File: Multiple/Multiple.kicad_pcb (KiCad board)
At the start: 2 copper layers, 23.1 x 128.4 mm, 17 parts

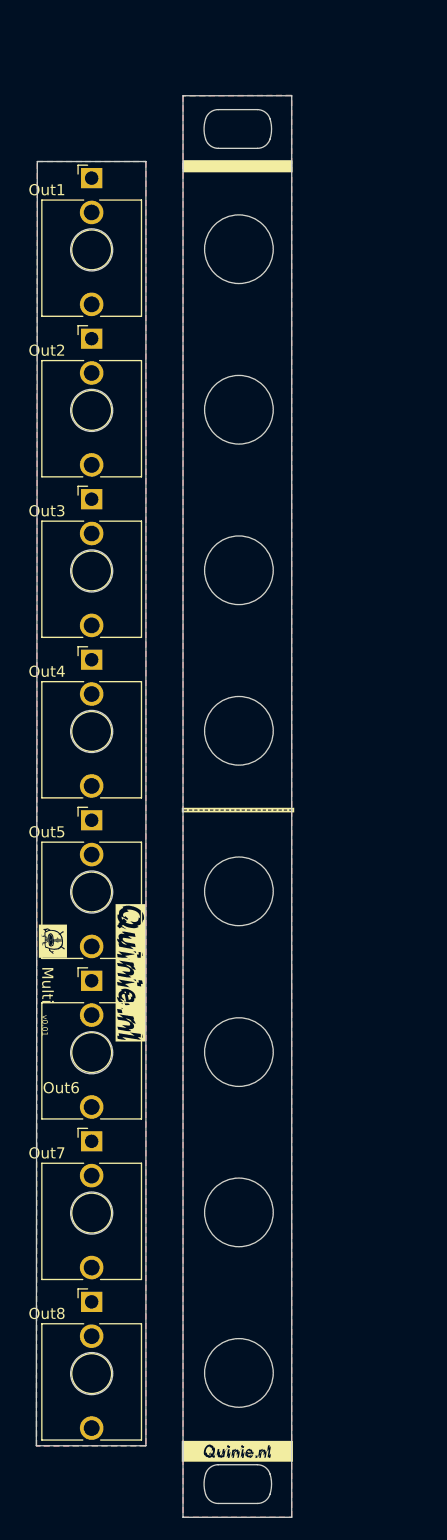
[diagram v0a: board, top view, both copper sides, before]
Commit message: Updates
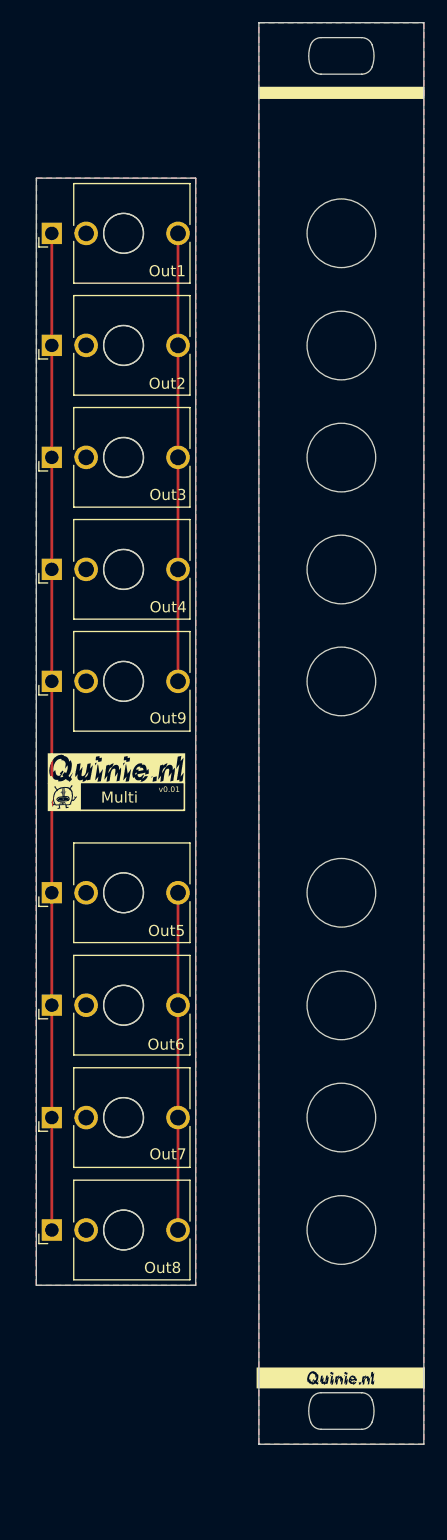
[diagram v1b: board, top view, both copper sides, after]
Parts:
- removed the kibuzzard-63663374 at (30.5, 108.9)
- removed the kibuzzard-63663374 at (37.6, 108.9)
- removed the kibuzzard-63663374 at (50.6, 108.7)
- removed the kibuzzard-63729A5C at (37.5, 111.8)
- removed the kibuzzard-63729A5C at (30.5, 111.8)
- removed the kibuzzard-63729A5C at (43.6, 111.5)
- removed kibuzzard-6564E26E: G***, kibuzzard-6564E26E
- removed kibuzzard-6564E2EE: G***, kibuzzard-6564E2EE
- removed kibuzzard-6564E9E6: G***, kibuzzard-6564E9E6
- added Out9: AudioJack2_SwitchT, Connector_Audio:Jack_3.5mm_QingPu_WQP-PJ398SM_Vertical_CircularHoles, F.Cu at (30.4, 85.5)
- added REF**: ESD-Logo_6.6x6mm_SilkScreen, Symbol:ESD-Logo_6.6x6mm_SilkScreen, B.Cu at (60.2, 109.6)
- added REF**: KiCad-Logo2_5mm_SilkScreen, Symbol:KiCad-Logo2_5mm_SilkScreen, B.Cu at (52.1, 95.0)
- added REF**: WEEE-Logo_4.2x6mm_SilkScreen, Symbol:WEEE-Logo_4.2x6mm_SilkScreen, B.Cu at (58.6, 91.4)
- added REF**: OSHW-Logo2_7.3x6mm_SilkScreen, Symbol:OSHW-Logo2_7.3x6mm_SilkScreen, B.Cu at (58.6, 97.5)
- added kibuzzard-63663374: G***, kibuzzard-63663374, F.Cu at (31.5, 95.9)
- added kibuzzard-63663374: G***, kibuzzard-63663374, B.Cu at (40.7, 95.7)
- added kibuzzard-63729A5C: G***, kibuzzard-63729A5C, F.Cu at (36.2, 93.3)
- added kibuzzard-63729A5C: G***, kibuzzard-63729A5C, B.Cu at (36.0, 93.1)
- added kibuzzard-656B6089: G***, kibuzzard-656B6089, F.Cu at (56.6, 146.1)
- added kibuzzard-656B60C2: G***, kibuzzard-656B60C2, F.Cu at (56.5, 148.4)
- added kibuzzard-656B617B: G***, kibuzzard-656B617B, B.Cu at (56.5, 38.1)
- moved Out4 8.92 mm to (30.4, 75.3), turned to 90 degrees
- moved Out5 7.47 mm to (30.4, 104.5), turned to 90 degrees
- moved Out8 7.42 mm to (30.4, 135.0), turned to 90 degrees
- moved Out1 6.15 mm to (30.4, 45.0), turned to 90 degrees
- moved Out3 5.22 mm to (30.4, 65.2), turned to 90 degrees
- moved Out6 4.22 mm to (30.4, 114.7), turned to 90 degrees
- moved Out7 4.19 mm to (30.4, 124.9), turned to 90 degrees
- moved Out2 3.65 mm to (30.4, 55.1), turned to 90 degrees
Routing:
- net GND: track 0.00 -> 90.0 mm
- net Net-(Out1-PadT): track 0.00 -> 40.5 mm
- net Net-(Out5-PadT): track 0.00 -> 30.5 mm
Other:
- board size 23.1 x 128.4 mm -> 35 x 128.4 mm
- board text added: "JLCJLCJLCJLC"
